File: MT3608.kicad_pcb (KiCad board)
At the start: 2 copper layers, 40 x 20 mm, 19 parts, among them J1 IN, J2 OUT, U1 MT3608

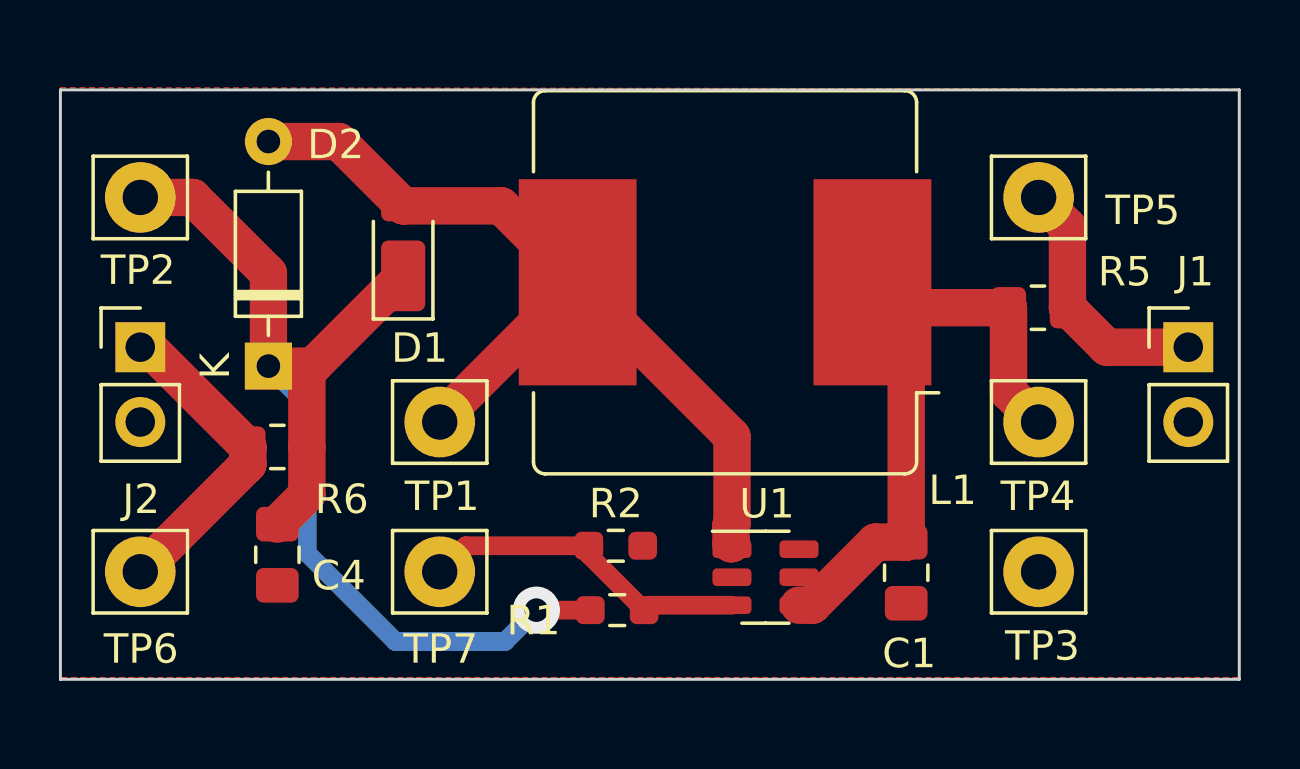
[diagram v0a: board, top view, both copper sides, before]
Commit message: Take 2
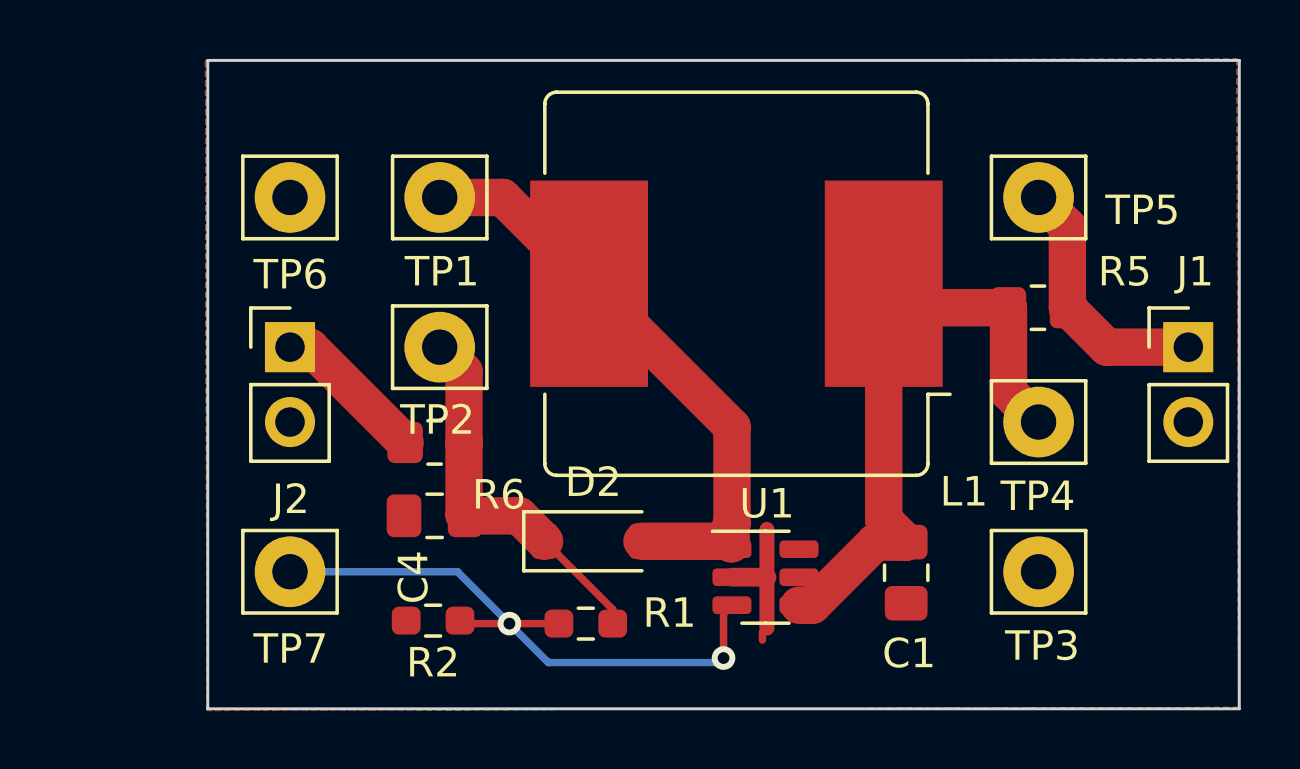
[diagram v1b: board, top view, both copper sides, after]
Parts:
- removed D1: SBR3U, Diode_SMD:D_PowerDI-123
- D2: value 1N4148 -> MBR0540; footprint Diode_THT:D_DO-35_SOD27_P7.62mm_Horizontal -> Diode_SMD:D_SOD-123
- moved TP6 13.7 mm to (102.8, 103.7)
- moved D2 12.5 mm to (113.1, 115.3), turned to 0 degrees
- moved TP2 11.4 mm to (107.9, 108.7)
- moved TP1 7.62 mm to (107.9, 103.7)
- moved R2 6.70 mm to (107.6, 118.0), turned to 180 degrees
- moved C4 5.50 mm to (107.7, 114.5), turned to 180 degrees
- moved R6 5.34 mm to (107.7, 112.0)
- moved J2 5.08 mm to (102.8, 108.7)
- moved TP7 5.08 mm to (102.8, 116.3)
- moved R1 1.16 mm to (112.8, 118.1), turned to 180 degrees
- moved L1 0.39 mm to (117.9, 106.6)
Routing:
- net Net-(D2-K): track 38.5 -> 12.9 mm, vias 1 -> 0
- net Net-(D2-A): track 30.2 -> 20.2 mm
- net Net-(U1-FB): track 11.4 -> 21.4 mm, vias 0 -> 2
- net Net-(J2-Pin_1): track 10.8 -> 5.25 mm
- net GND: track 0.00 -> 5.01 mm
- net Net-(U1-EN): track 23.1 -> 25.3 mm
- added copper zone on B.Cu, net GND
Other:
- board size 40 x 20 mm -> 35 x 22 mm
